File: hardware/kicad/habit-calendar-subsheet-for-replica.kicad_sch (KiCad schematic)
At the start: 114 parts, among them J1 Conn_01x01, J10 Conn_01x01, J11 Conn_01x01, J12 Conn_01x01, J13 Conn_01x01, J14 Conn_01x01, J15 Conn_01x01, J16 Conn_01x01, J17 Conn_01x01, J18 Conn_01x01, J19 Conn_01x01, J2 Conn_01x01, J20 Conn_01x01, J21 Conn_01x01, J22 Conn_01x01, J23 Conn_01x01, J24 Conn_01x01, J25 Conn_01x01, J26 Conn_01x01, J27 Conn_01x01, J28 Conn_01x01, J29 Conn_01x01, J3 Conn_01x01, J30 Conn_01x01, J31 Conn_01x01, J4 Conn_01x01, J5 Conn_01x01, J51 Conn_01x01, J6 Conn_01x01, J60 Conn_01x01, J63 Conn_01x01, J64 Conn_01x01, J65 Conn_01x01, J66 Conn_01x01, J67 Conn_01x01, J68 Conn_01x01, J69 Conn_01x01, J7 Conn_01x01, J70 Conn_01x01, J71 Conn_01x01, J72 Conn_01x01, J73 Conn_01x01, J74 Conn_01x01, J75 Conn_01x01, J76 Conn_01x01, J77 Conn_01x01, J78 Conn_01x01, J8 Conn_01x01, J9 Conn_01x01, SW1 TS-1187A-B-A-B, SW10 TS-1187A-B-A-B, SW11 TS-1187A-B-A-B, SW12 TS-1187A-B-A-B, SW2 TS-1187A-B-A-B, SW3 TS-1187A-B-A-B, SW4 TS-1187A-B-A-B, SW5 TS-1187A-B-A-B, SW6 TS-1187A-B-A-B, SW7 TS-1187A-B-A-B, SW8 TS-1187A-B-A-B, SW9 TS-1187A-B-A-B, U1 PY32F002AF15P6TU

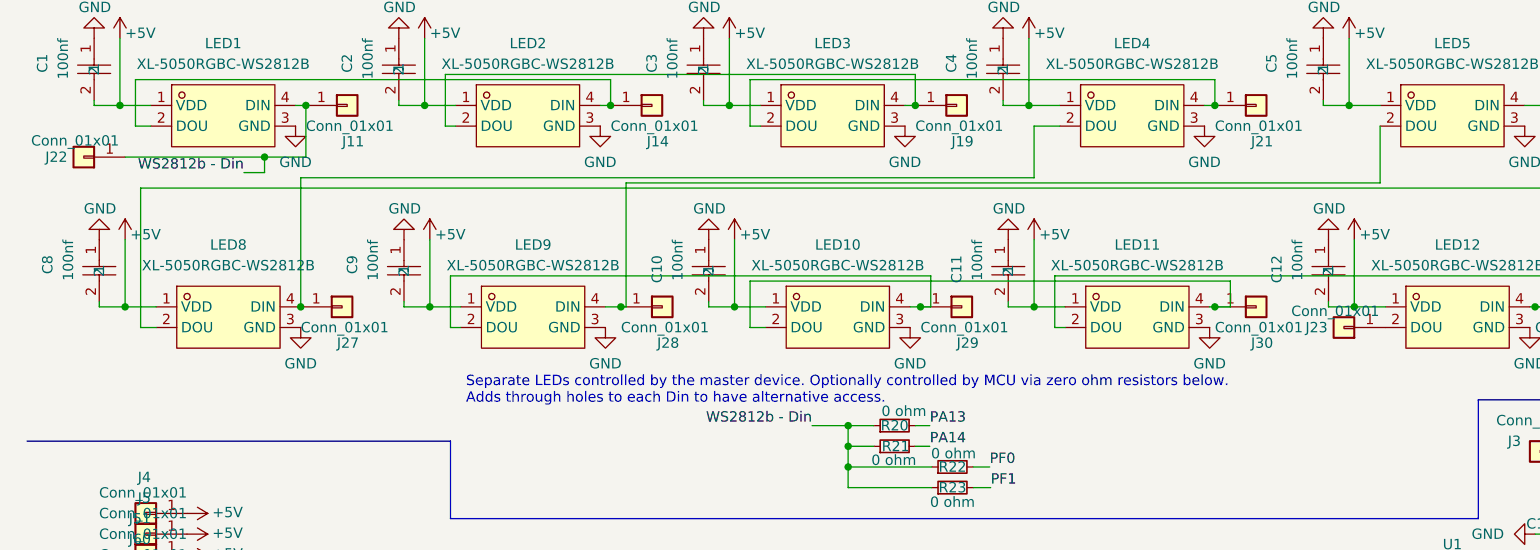
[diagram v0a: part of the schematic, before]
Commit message: Sent to production!
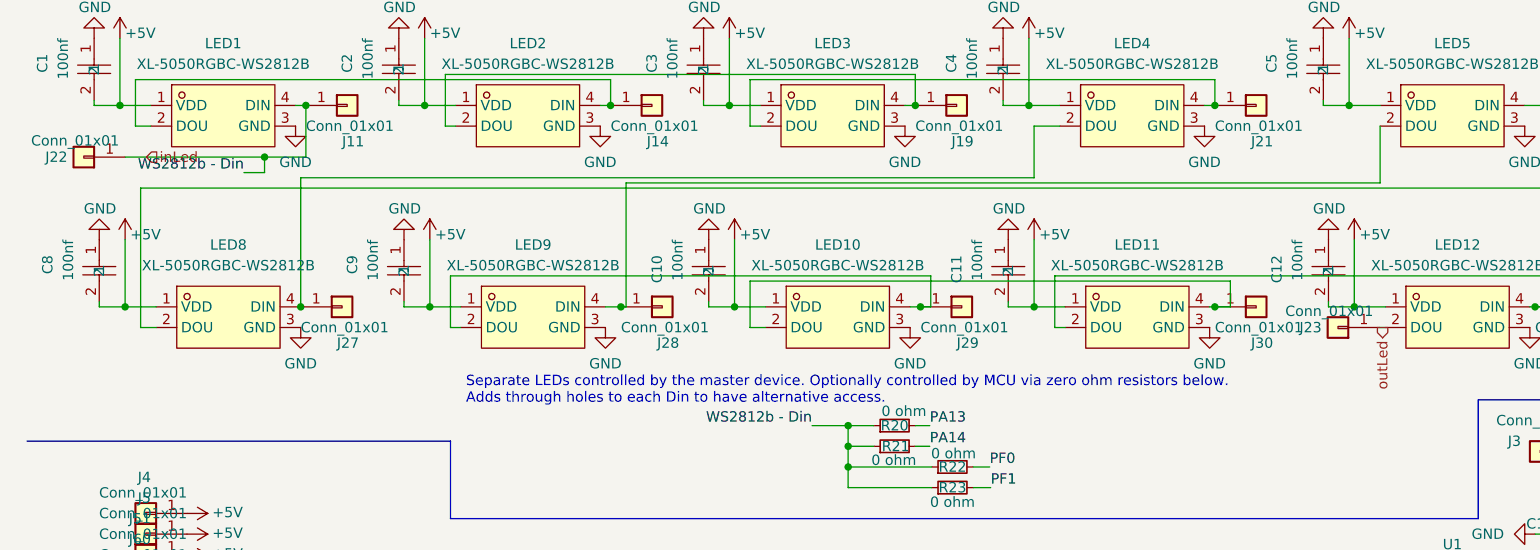
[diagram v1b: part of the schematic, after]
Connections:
- net outLed: now reaches J23.1 (Pin_1), LED12.2 (DOU)
- net WS2812b - Din renamed inLed
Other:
- moved on the sheet: J23
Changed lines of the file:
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@@
+    (stroke (width 0) (type default) (color 0 0 0 0))
+  )
+  (wire (pts (xy 179.6034 55.245) (xy 180.34 55.245))
     (stroke (width 0) (type default) (color 0 0 0 0))
   )
@@
     (effects (font (size 1.27 1.27)) (justify right))
   )
+  (hierarchical_label "outLed" (shape output) (at 180.0098 55.245 270)
+    (effects (font (size 1.27 1.27)) (justify right))
+  )
   (hierarchical_label "outPF0" (shape input) (at 30.099 142.0876 270)
     (effects (font (size 1.27 1.27)) (justify right))
@@
   (hierarchical_label "outPF1" (shape input) (at 31.7754 142.113 270)
     (effects (font (size 1.27 1.27)) (justify right))
+  )
+  (hierarchical_label "inLed" (shape input) (at 28.0162 34.29 0)
+    (effects (font (size 1.27 1.27)) (justify left))
   )
   (hierarchical_label "inPF0" (shape input) (at 35.2044 98.4504 0)
@@
     (pin "1")
   )
-  (symbol (lib_id "Connector_Generic:Conn_01x01") (at 175.26 55.245 180) (unit 1)
-    (in_bom yes) (on_board yes)
-    (property "Reference" "J23" (id 0) (at 173.2534 55.245 0)
-      (effects (font (size 1.27 1.27)) (justify left))
-    )
-    (property "Value" "Conn_01x01" (id 1) (at 179.6034 53.2384 0)
-      (effects (font (size 1.27 1.27)) (justify left))
-    )
-    (property "Footprint" "Connector_PinHeader_2.54mm:PinHeader_1x01_P2.54mm_Vertical" (id 2) (at 175.26 55.245 0)
-      (effects (font (size 1.27 1.27)) hide)
-    )
-    (property "Datasheet" "~" (id 3) (at 175.26 55.245 0)
-      (effects (font (size 1.27 1.27)) hide)
-    )
+  (symbol (lib_id "Connector_Generic:Conn_01x01") (at 174.5234 55.245 180) (unit 1)
+    (in_bom yes) (on_board yes)
+    (property "Reference" "J23" (id 0) (at 172.5168 55.245 0)
+      (effects (font (size 1.27 1.27)) (justify left))
+    )
+    (property "Value" "Conn_01x01" (id 1) (at 178.8668 53.2384 0)
+      (effects (font (size 1.27 1.27)) (justify left))
+    )
+    (property "Footprint" "Connector_PinHeader_2.54mm:PinHeader_1x01_P2.54mm_Vertical" (id 2) (at 174.5234 55.245 0)
+      (effects (font (size 1.27 1.27)) hide)
+    )
+    (property "Datasheet" "~" (id 3) (at 174.5234 55.245 0)
+      (effects (font (size 1.27 1.27)) hide)
+    )
